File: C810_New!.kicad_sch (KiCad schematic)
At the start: 79 parts, among them J1 Conn_01x03, J2 Conn_01x04, J20 Conn_01x07, J3 Conn_ST_STDC14, J4 USB_C_Receptacle_USB2.0_16P, Q1 BSC159N10LSFG, Q2 BSC159N10LSFG, Q3 BSC159N10LSFG, Q4 BSC159N10LSFG, Q5 BSC159N10LSFG, Q6 BSC159N10LSFG, SW1 button, U1 IR2302, U10 L7812, U11 3.3, U12 Regulator_5.0, U2 IR2302, U3 IR2302, U4 STM32F303K8Tx, U5 NCS214, U6 NCS214, U8 MCP2561-E-SN, Y2 16MHz

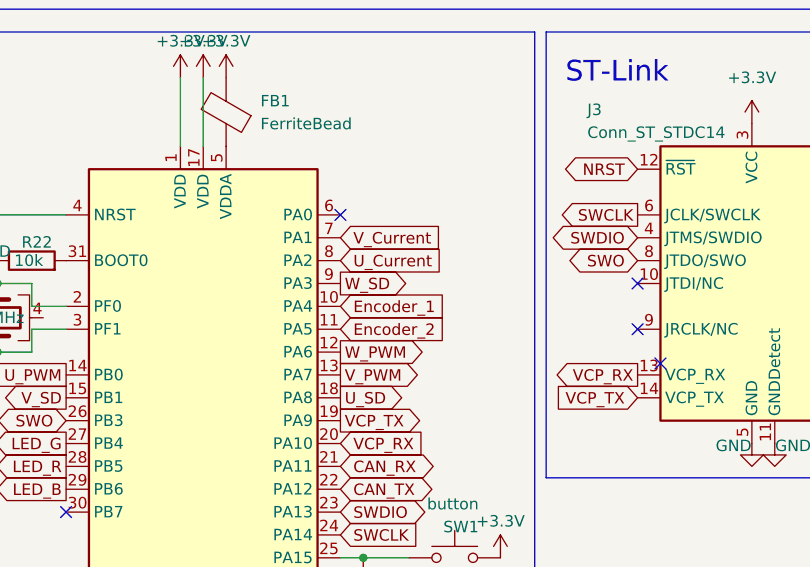
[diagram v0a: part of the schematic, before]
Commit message: 配線が無理すぎるので寝る
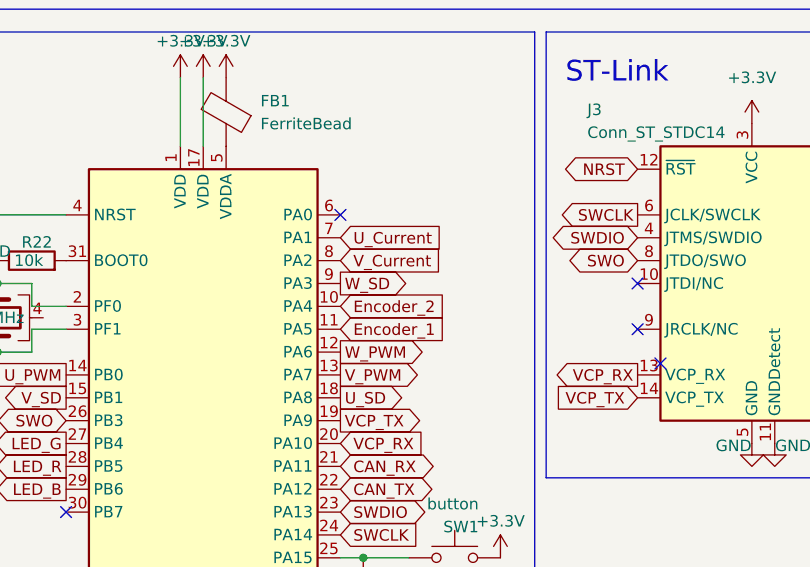
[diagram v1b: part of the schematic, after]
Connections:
- net Encoder_1: now also U4.11 (PA5); no longer U4.10 (PA4)
- net Encoder_2: now also U4.10 (PA4); no longer U4.11 (PA5)
- net U_Current: now also U4.7 (PA1); no longer U4.8 (PA2)
- net V_Current: now also U4.8 (PA2); no longer U4.7 (PA1)
